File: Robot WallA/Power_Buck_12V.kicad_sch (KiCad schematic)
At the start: 19 parts, among them Q3 BSS138

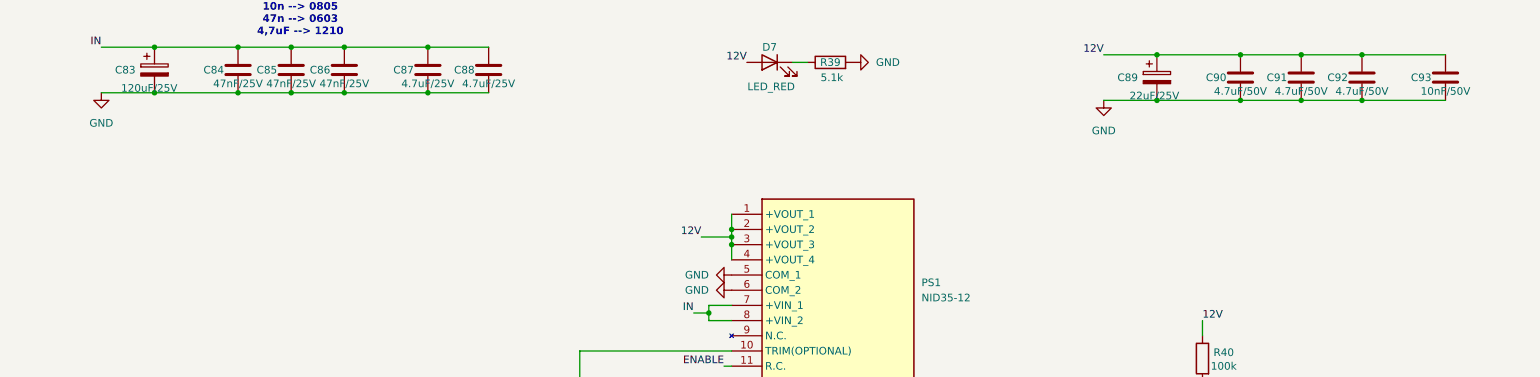
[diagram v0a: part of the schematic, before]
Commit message: Continue to route
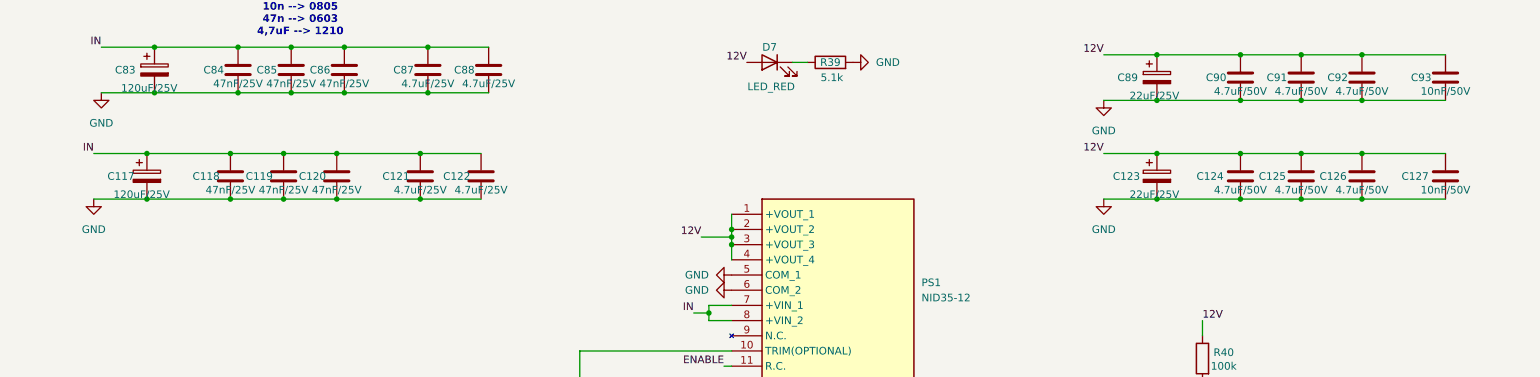
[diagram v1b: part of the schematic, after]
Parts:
- added C117: 120uF/25V, SamacSys_Parts:EEE0JA331XP, symbol Device:C_Polarized
- added C118, C119, C120: 47nF/25V, Capacitor_SMD:C_0603_1608Metric_Pad1.08x0.95mm_HandSolder, symbol Device:C
- added C121, C122: 4.7uF/25V, Capacitor_SMD:C_1210_3225Metric_Pad1.33x2.70mm_HandSolder, symbol Device:C
- added C123: 22uF/25V, SamacSys_Parts:EEE1AA220WR, symbol Device:C_Polarized
- added C124, C125, C126: 4.7uF/50V, Capacitor_SMD:C_0805_2012Metric_Pad1.18x1.45mm_HandSolder, symbol Device:C
- added C127: 10nF/50V, Capacitor_SMD:C_0805_2012Metric_Pad1.18x1.45mm_HandSolder, symbol Device:C
- C89: footprint Capacitor_SMD:C_0805_2012Metric_Pad1.18x1.45mm_HandSolder -> SamacSys_Parts:EEE1AA220WR; Height (none) -> 5.5; Manufacturer_Part_Number (none) -> EEE-FN1E220R
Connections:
- net GND: now also C117.2, C118.2, C119.2, C120.2, C121.2, C122.2, C123.2, C124.2, C125.2, C126.2, C127.2
- net IN: now also C117.1, C118.1, C119.1, C120.1, C121.1, C122.1
- net OUT: now also C123.1, C124.1, C125.1, C126.1, C127.1

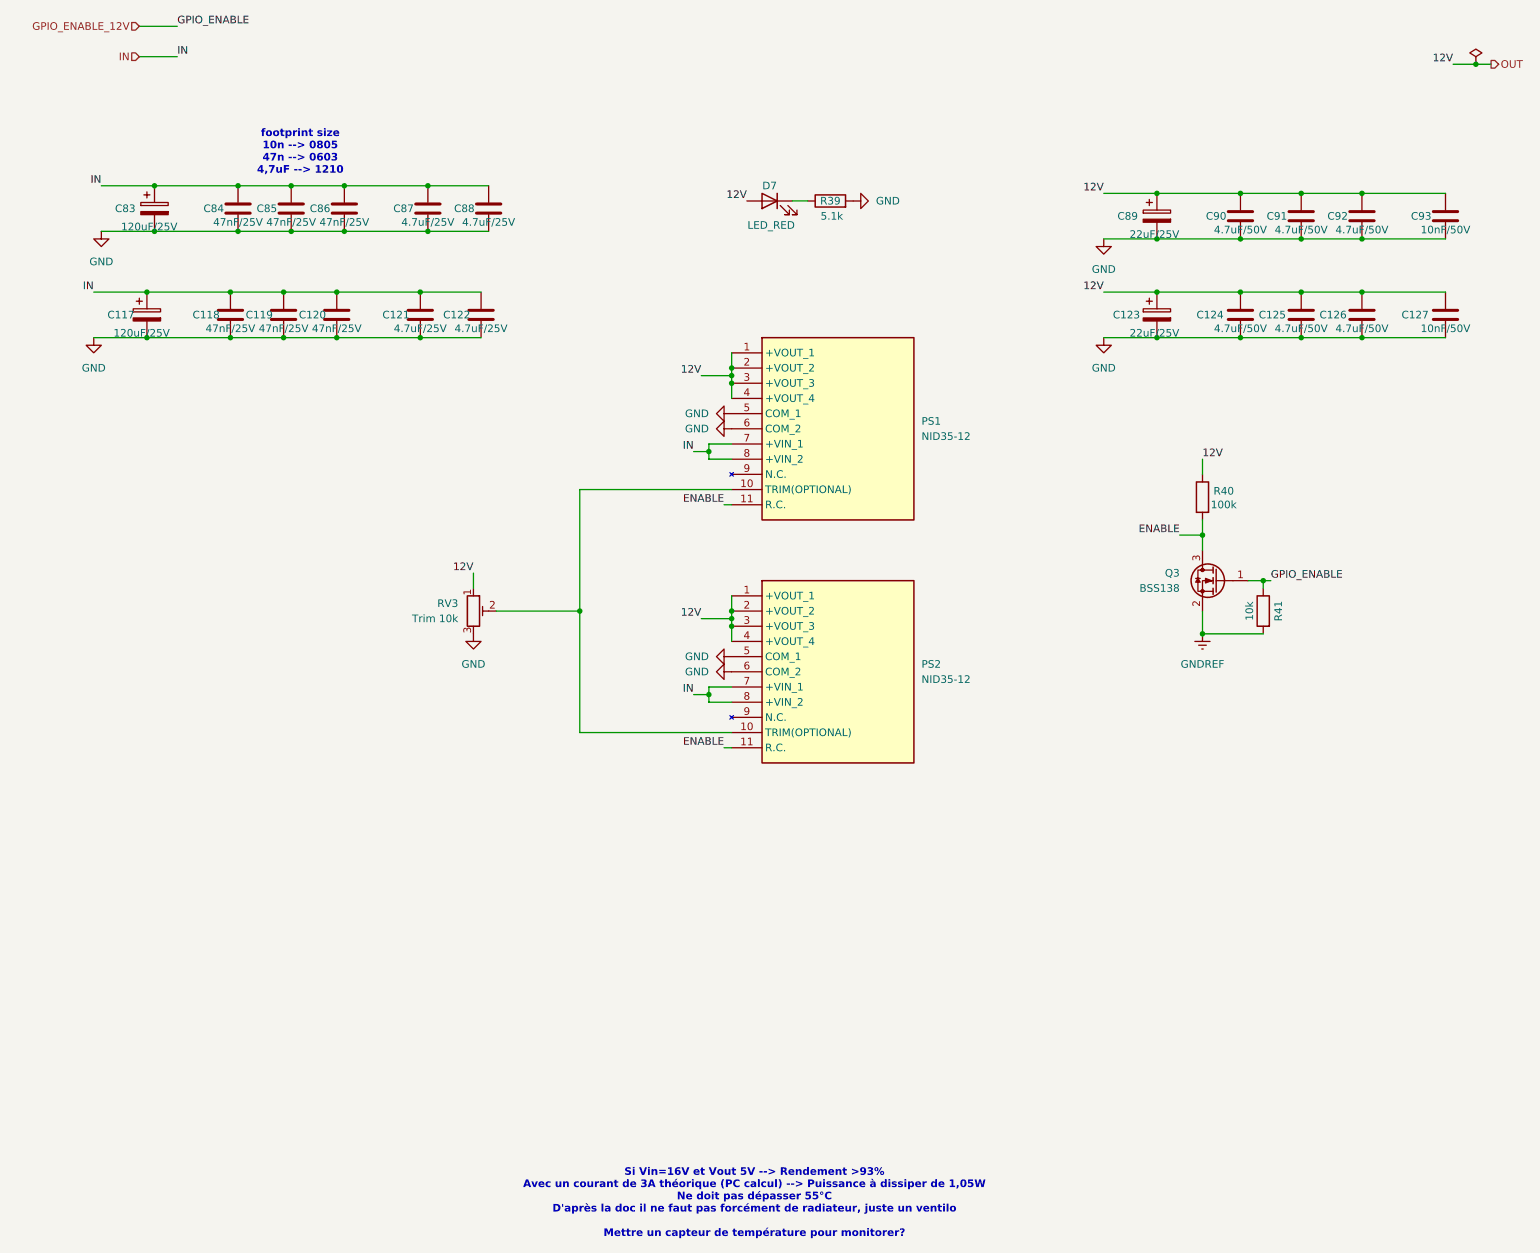
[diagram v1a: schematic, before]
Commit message: Reworked 12V and 5V power supplies, continue routing
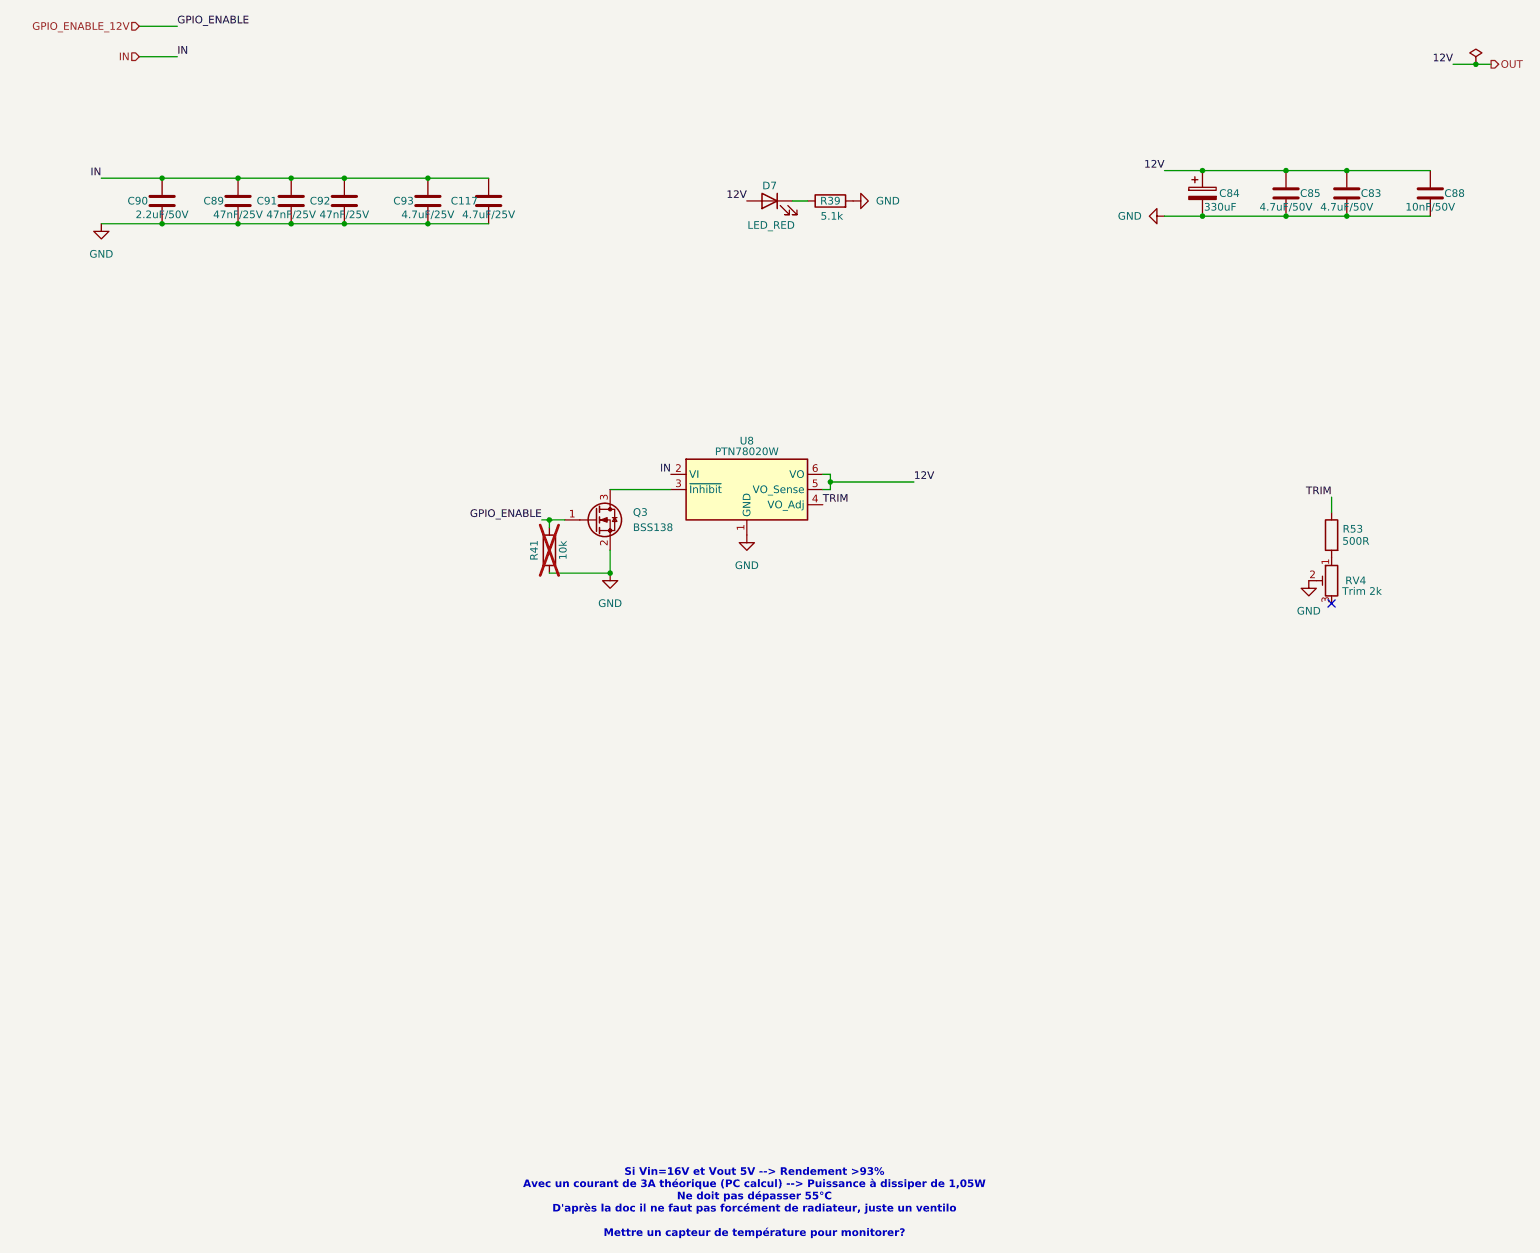
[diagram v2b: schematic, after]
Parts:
- removed C117, C83: 120uF/25V, SamacSys_Parts:EEE0JA331XP, symbol Device:C_Polarized
- removed C118, C119, C120, C84, C86: 47nF/25V, Capacitor_SMD:C_0603_1608Metric_Pad1.08x0.95mm_HandSolder, symbol Device:C
- removed C121, C122, C87: 4.7uF/25V, Capacitor_SMD:C_1210_3225Metric_Pad1.33x2.70mm_HandSolder, symbol Device:C
- removed C123, C89: 22uF/25V, SamacSys_Parts:EEE1AA220WR, symbol Device:C_Polarized
- removed C124, C125, C126: 4.7uF/50V, Capacitor_SMD:C_0805_2012Metric_Pad1.18x1.45mm_HandSolder, symbol Device:C
- removed C127: 10nF/50V, Capacitor_SMD:C_0805_2012Metric_Pad1.18x1.45mm_HandSolder, symbol Device:C
- removed PS1, PS2: NID35-12, SamacSys_Parts:NID3512, symbol SamacSys_new:NID35-12
- removed R40: 100k, Resistor_SMD:R_0603_1608Metric_Pad0.98x0.95mm_HandSolder, symbol Device:R
- removed RV3: Trim 10k, SamacSys_Parts:TC33X2503E, symbol Device:R_Potentiometer_Trim
- added C117: 4.7uF/25V, Capacitor_SMD:C_1210_3225Metric_Pad1.33x2.70mm_HandSolder, symbol Device:C
- added C83: 4.7uF/50V, Capacitor_SMD:C_1210_3225Metric_Pad1.33x2.70mm_HandSolder, symbol Device:C
- added C84: 330uF, SamacSys_Parts:CAPPRD500W65D1000H1800, symbol Device:C_Polarized
- added C89: 47nF/25V, Capacitor_SMD:C_0603_1608Metric_Pad1.08x0.95mm_HandSolder, symbol Device:C
- added R53: 500R, Resistor_SMD:R_0603_1608Metric_Pad0.98x0.95mm_HandSolder, symbol Device:R
- added RV4: Trim 2k, SamacSys_Parts:TC42X2202E, symbol Device:R_Potentiometer_Trim
- added U8: PTN78020W, Module:Texas_EUK_R-PDSS-T7_THT, symbol Converter_DCDC:PTN78020W_EUK-7
- C85: value 47nF/25V -> 4.7uF/50V; footprint Capacitor_SMD:C_0603_1608Metric_Pad1.08x0.95mm_HandSolder -> Capacitor_SMD:C_1210_3225Metric_Pad1.33x2.70mm_HandSolder; Manufacturer_Part_Number (none) -> GRM32ER71H475KA88L
- C88: value 4.7uF/25V -> 10nF/50V; footprint Capacitor_SMD:C_1210_3225Metric_Pad1.33x2.70mm_HandSolder -> Capacitor_SMD:C_0805_2012Metric_Pad1.18x1.45mm_HandSolder
- C90: value 4.7uF/50V -> 2.2uF/50V; footprint Capacitor_SMD:C_0805_2012Metric_Pad1.18x1.45mm_HandSolder -> Capacitor_SMD:C_1210_3225Metric_Pad1.33x2.70mm_HandSolder; Manufacturer_Part_Number (none) -> C3225X7R1H225K250AB
- C91, C92: value 4.7uF/50V -> 47nF/25V; footprint Capacitor_SMD:C_0805_2012Metric_Pad1.18x1.45mm_HandSolder -> Capacitor_SMD:C_0603_1608Metric_Pad1.08x0.95mm_HandSolder
- C93: value 10nF/50V -> 4.7uF/25V; footprint Capacitor_SMD:C_0805_2012Metric_Pad1.18x1.45mm_HandSolder -> Capacitor_SMD:C_1210_3225Metric_Pad1.33x2.70mm_HandSolder; Manufacturer_Part_Number (none) -> GRM32ER71H475KA88L
- R41: now not fitted
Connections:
- net GNDREF is gone; now on net GND: Q3.2 (S), R41.2
- net GND: now also C117.2, C83.2, C84.2, C89.2, RV4.2, U8.1 (GND), U8.7 (GND)
- net IN: now also C90.1, C91.1, C92.1, C93.1, C117.1, C89.1, U8.2 (VI); no longer C85.1, C88.1
- net OUT: now also C85.1, C88.1, C83.1, C84.1, U8.5 (VO_Sense), U8.6 (VO); no longer C90.1, C91.1, C92.1, C93.1
- net ENABLE: no longer names the net of Q3.3 (D)
- net ENABLE: now also U8.3 (~{Inhibit})
- new net: R53.2, RV4.1
- new net TRIM: R53.1, U8.4 (VO_Adj)
- no-connect marks 0 -> 1
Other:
- note removed: "footprint size 10n --> 0805 47n --> 0603 4,7uF --> 1210"
- moved on the sheet: C90, Q3
